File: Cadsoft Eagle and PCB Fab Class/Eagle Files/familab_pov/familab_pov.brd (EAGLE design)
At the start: 58.4 x 42.9 mm, 7 parts, among them U1 Tiny85-20-SMT

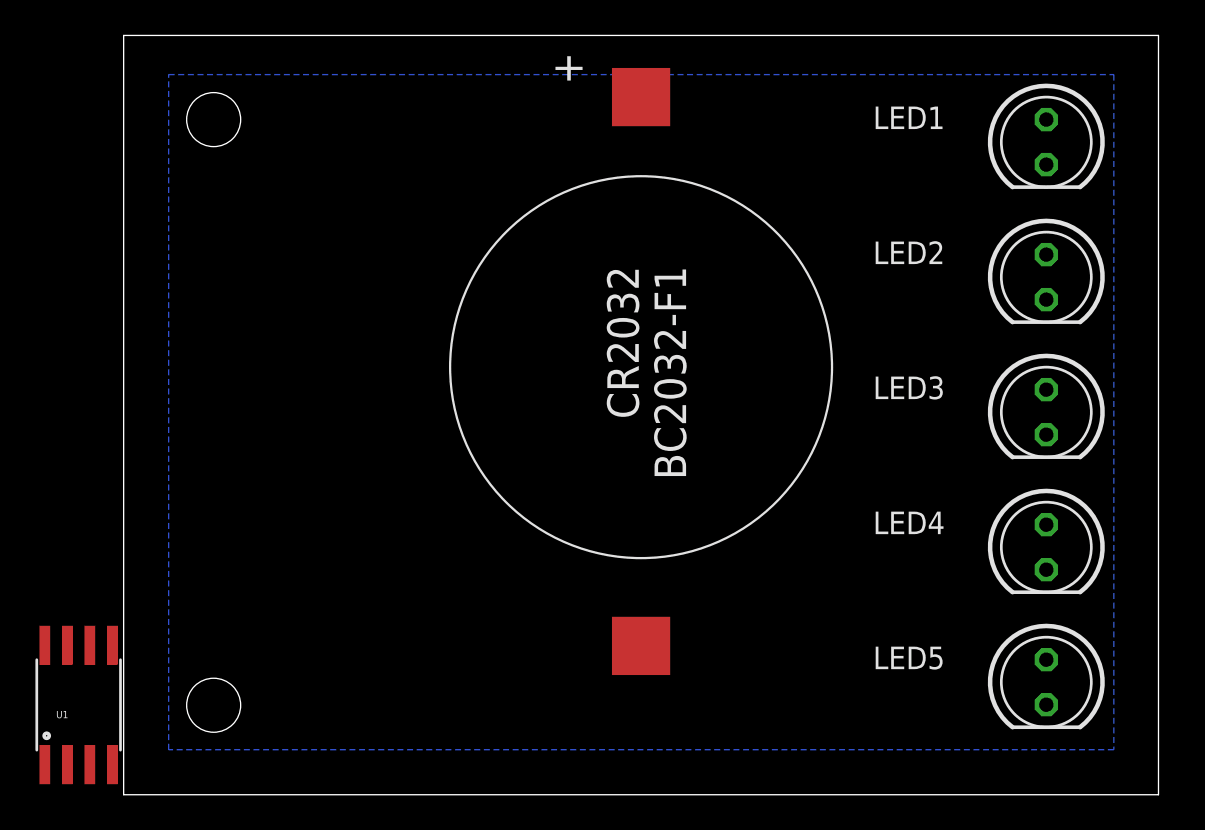
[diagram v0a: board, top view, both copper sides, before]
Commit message: Updates
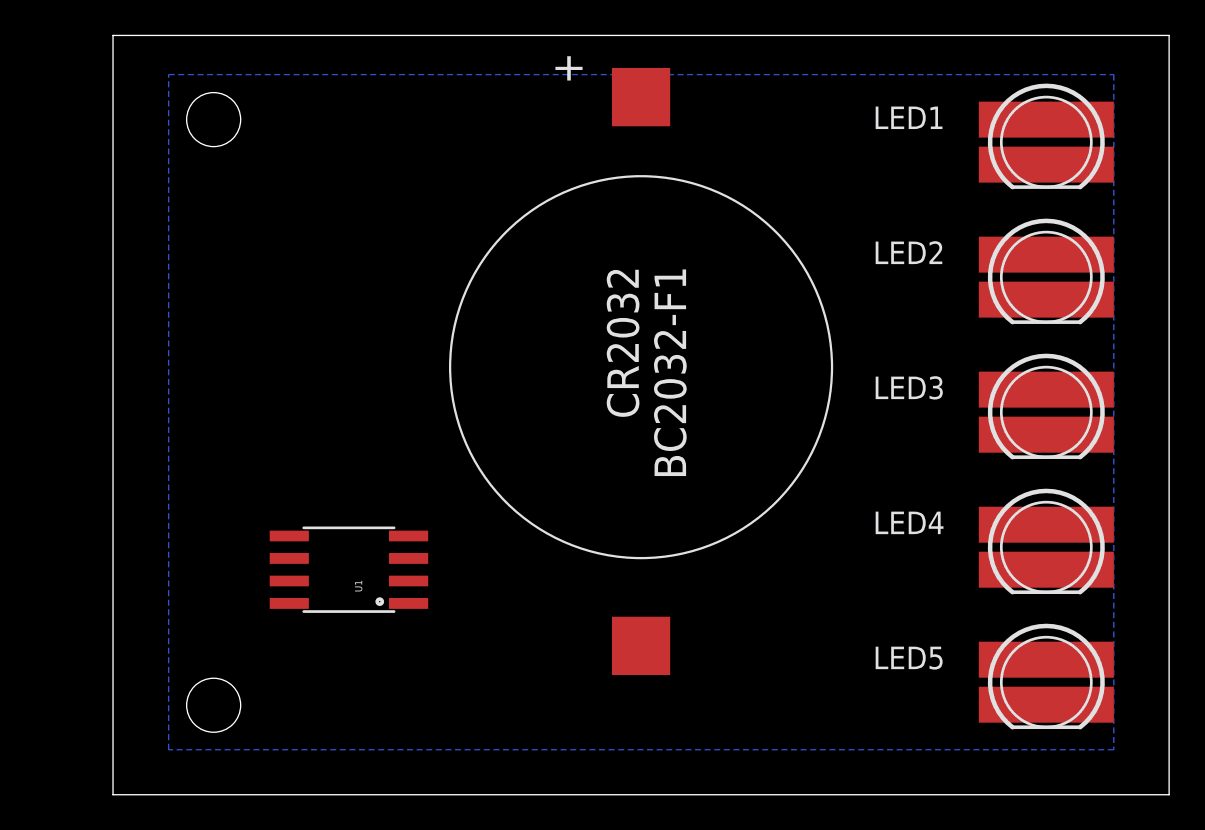
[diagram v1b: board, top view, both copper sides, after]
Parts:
- LED1, LED2, LED3, LED4, LED5: device led:LED5MM -> led:LED5MM_SMD_SIDE
- moved U1 17.0 mm to (12.7, 12.7), turned to 90 degrees
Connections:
- net N$1 renamed PB0
- net N$7 renamed PB5
- removed net N$10: LED5.A
- removed net N$2: U1.6
- removed net N$3: LED1.A
- removed net N$4: U1.7
- removed net N$5: U1.2
- removed net N$6: U1.3
- removed net N$8: LED2.A
- removed net N$9: LED4.A
- new net PB1: LED2.A, U1.6
- new net PB2: LED1.A, U1.7
- new net PB3: LED5.A, U1.2
- new net PB4: LED4.A, U1.3
- net GND: now also LED1.C, LED2.C, LED3.C, LED4.C, LED5.C; no longer LED1.K, LED2.K, LED3.K, LED4.K, LED5.K
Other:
- board size 58.4 x 42.9 mm -> 59.6 x 42.9 mm
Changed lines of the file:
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@@
 <layer number="113" name="IDFDebug" color="7" fill="1" visible="yes" active="yes"/>
 <layer number="116" name="Patch_BOT" color="9" fill="4" visible="yes" active="yes"/>
+<layer number="117" name="mPads" color="7" fill="1" visible="no" active="no"/>
+<layer number="118" name="Rect_Pads" color="7" fill="1" visible="yes" active="yes"/>
+<layer number="119" name="mUnrouted" color="7" fill="1" visible="no" active="no"/>
+<layer number="120" name="mDimension" color="7" fill="1" visible="no" active="no"/>
 <layer number="121" name="_tsilk" color="7" fill="1" visible="yes" active="yes"/>
 <layer number="122" name="_bsilk" color="7" fill="1" visible="yes" active="yes"/>
@@
 <layer number="127" name="_tValues" color="7" fill="1" visible="yes" active="yes"/>
 <layer number="128" name="_bValues" color="7" fill="1" visible="yes" active="yes"/>
+<layer number="129" name="mtStop" color="7" fill="1" visible="no" active="no"/>
+<layer number="130" name="mbStop" color="7" fill="1" visible="no" active="no"/>
 <layer number="131" name="tAdjust" color="7" fill="1" visible="yes" active="yes"/>
 <layer number="132" name="bAdjust" color="7" fill="1" visible="yes" active="yes"/>
+<layer number="133" name="mtFinish" color="7" fill="1" visible="no" active="no"/>
+<layer number="134" name="mbFinish" color="7" fill="1" visible="no" active="no"/>
+<layer number="135" name="mtGlue" color="7" fill="1" visible="no" active="no"/>
+<layer number="136" name="mbGlue" color="7" fill="1" visible="no" active="no"/>
+<layer number="137" name="mtTest" color="7" fill="1" visible="no" active="no"/>
+<layer number="138" name="mbTest" color="7" fill="1" visible="no" active="no"/>
+<layer number="139" name="mtKeepout" color="7" fill="1" visible="no" active="no"/>
+<layer number="140" name="mbKeepout" color="7" fill="1" visible="no" active="no"/>
+<layer number="141" name="mtRestrict" color="7" fill="1" visible="no" active="no"/>
+<layer number="142" name="mbRestrict" color="7" fill="1" visible="no" active="no"/>
+<layer number="143" name="mvRestrict" color="7" fill="1" visible="no" active="no"/>
 <layer number="144" name="Drill_legend" color="7" fill="1" visible="yes" active="yes"/>
+<layer number="145" name="mHoles" color="7" fill="1" visible="no" active="no"/>
+<layer number="146" name="mMilling" color="7" fill="1" visible="no" active="no"/>
+<layer number="147" name="mMeasures" color="7" fill="1" visible="no" active="no"/>
+<layer number="148" name="mDocument" color="7" fill="1" visible="no" active="no"/>
+<layer number="149" name="mReference" color="7" fill="1" visible="no" active="no"/>
 <layer number="150" name="Notes" color="7" fill="1" visible="yes" active="yes"/>
 <layer number="151" name="HeatSink" color="7" fill="1" visible="yes" active="yes"/>
@@
 <layer number="154" name="FabDoc2" color="7" fill="1" visible="yes" active="yes"/>
 <layer number="155" name="FabDoc3" color="7" fill="1" visible="yes" active="yes"/>
+<layer number="191" name="mNets" color="7" fill="1" visible="no" active="no"/>
+<layer number="192" name="mBusses" color="7" fill="1" visible="no" active="no"/>
+<layer number="193" name="mPins" color="7" fill="1" visible="no" active="no"/>
+<layer number="194" name="mSymbols" color="7" fill="1" visible="no" active="no"/>
+<layer number="195" name="mNames" color="7" fill="1" visible="no" active="no"/>
+<layer number="196" name="mValues" color="7" fill="1" visible="no" active="no"/>
 <layer number="199" name="Contour" color="7" fill="1" visible="yes" active="yes"/>
 <layer number="200" name="200bmp" color="1" fill="10" visible="yes" active="yes"/>
@@
 <layer number="223" name="223bmp" color="24" fill="1" visible="no" active="no"/>
 <layer number="224" name="224bmp" color="25" fill="1" visible="no" active="no"/>
+<layer number="231" name="Eagle3D_PG1" color="7" fill="1" visible="no" active="no"/>
+<layer number="232" name="Eagle3D_PG2" color="7" fill="1" visible="no" active="no"/>
+<layer number="233" name="Eagle3D_PG3" color="7" fill="1" visible="no" active="no"/>
 <layer number="248" name="Housing" color="7" fill="1" visible="yes" active="yes"/>
 <layer number="249" name="Edge" color="7" fill="1" visible="yes" active="yes"/>
@@
 <board>
 <plain>
-<wire x1="0" y1="0" x2="58.4" y2="0" width="0" layer="20"/>
-<wire x1="58.4" y1="0" x2="58.4" y2="42.85" width="0" layer="20"/>
-<wire x1="58.4" y1="42.85" x2="0" y2="42.85" width="0" layer="20"/>
-<wire x1="0" y1="42.85" x2="0" y2="0" width="0" layer="20"/>
+<wire x1="-0.6" y1="0" x2="59" y2="0" width="0" layer="20"/>
+<wire x1="59" y1="0" x2="59" y2="42.85" width="0" layer="20"/>
+<wire x1="59" y1="42.85" x2="-0.6" y2="42.85" width="0" layer="20"/>
+<wire x1="-0.6" y1="42.85" x2="-0.6" y2="0" width="0" layer="20"/>
 <hole x="5.08" y="5.05" drill="3.048"/>
 <hole x="5.08" y="38.1" drill="3.048"/>
@@
 </autorouter>
 <elements>
-<element name="LED1" library="led" package="LED5MM" value="" x="52.07" y="36.83" smashed="yes" rot="R270">
+<element name="LED1" library="led" package="LED5MM_SMD_SIDE" value="" x="52.07" y="36.83" smashed="yes" rot="R270">
 <attribute name="NAME" x="46.355" y="38.8366" size="1.27" layer="25" ratio="10" rot="R180"/>
 <attribute name="VALUE" x="50.2666" y="33.6296" size="1.27" layer="27" ratio="10" rot="R270"/>
 </element>
-<element name="LED2" library="led" package="LED5MM" value="" x="52.07" y="29.21" smashed="yes" rot="R270">
+<element name="LED2" library="led" package="LED5MM_SMD_SIDE" value="" x="52.07" y="29.21" smashed="yes" rot="R270">
 <attribute name="NAME" x="46.355" y="31.2166" size="1.27" layer="25" ratio="10" rot="R180"/>
 <attribute name="VALUE" x="50.2666" y="26.0096" size="1.27" layer="27" ratio="10" rot="R270"/>
 </element>
-<element name="LED3" library="led" package="LED5MM" value="" x="52.07" y="21.59" smashed="yes" rot="R270">
+<element name="LED3" library="led" package="LED5MM_SMD_SIDE" value="" x="52.07" y="21.59" smashed="yes" rot="R270">
 <attribute name="NAME" x="46.355" y="23.5966" size="1.27" layer="25" ratio="10" rot="R180"/>
 <attribute name="VALUE" x="50.2666" y="18.3896" size="1.27" layer="27" ratio="10" rot="R270"/>
 </element>
-<element name="LED4" library="led" package="LED5MM" value="" x="52.07" y="13.97" smashed="yes" rot="R270">
+<element name="LED4" library="led" package="LED5MM_SMD_SIDE" value="" x="52.07" y="13.97" smashed="yes" rot="R270">
 <attribute name="NAME" x="46.355" y="15.9766" size="1.27" layer="25" ratio="10" rot="R180"/>
 <attribute name="VALUE" x="50.2666" y="10.7696" size="1.27" layer="27" ratio="10" rot="R270"/>
 </element>
-<element name="LED5" library="led" package="LED5MM" value="" x="52.07" y="6.35" smashed="yes" rot="R270">
+<element name="LED5" library="led" package="LED5MM_SMD_SIDE" value="" x="52.07" y="6.35" smashed="yes" rot="R270">
 <attribute name="NAME" x="46.355" y="8.3566" size="1.27" layer="25" ratio="10" rot="R180"/>
 <attribute name="VALUE" x="50.2666" y="3.1496" size="1.27" layer="27" ratio="10" rot="R270"/>
 </element>
 <element name="U$1" library="pov_class" package="CR2032_BC2032-F1" value="CR2032_HOLDER" x="29.2" y="39.37" rot="R270"/>
-<element name="U1" library="SparkFun-DigitalIC" package="SO08-EIAJ" value="Tiny85-20-SMT" x="-2.54" y="5.08">
-<attribute name="PROD_ID" value="IC-09092" x="-2.54" y="5.08" size="1.778" layer="27" display="off"/>
+<element name="U1" library="SparkFun-DigitalIC" package="SO08-EIAJ" value="Tiny85-20-SMT" x="12.7" y="12.7" rot="R90">
+<attribute name="PROD_ID" value="IC-09092" x="12.7" y="12.7" size="1.778" layer="27" rot="R90" display="off"/>
 </element>
 </elements>
 <signals>
 <signal name="GND">
-<contactref element="LED1" pad="K"/>
-<contactref element="LED2" pad="K"/>
-<contactref element="LED3" pad="K"/>
-<contactref element="LED4" pad="K"/>
-<contactref element="LED5" pad="K"/>
+<contactref element="LED1" pad="C"/>
+<contactref element="LED2" pad="C"/>
+<contactref element="LED3" pad="C"/>
+<contactref element="LED4" pad="C"/>
+<contactref element="LED5" pad="C"/>
 <polygon width="0.4064" layer="16">
 <vertex x="2.54" y="40.64"/>
@@
 <contactref element="U$1" pad="POS"/>
 </signal>
-<signal name="N$1">
+<signal name="PB0">
 <contactref element="U1" pad="5"/>
 <contactref element="LED3" pad="A"/>
-<wire x1="-0.635" y1="8.4328" x2="52.07" y2="22.86" width="0" layer="19" extent="1-1"/>
-</signal>
-<signal name="N$2">
+<wire x1="9.3472" y1="14.605" x2="52.07" y2="22.86" width="0" layer="19" extent="1-1"/>
+</signal>
+<signal name="PB1">
 <contactref element="U1" pad="6"/>
-</signal>
-<signal name="N$3">
+<contactref element="LED2" pad="A"/>
+<wire x1="9.3472" y1="13.335" x2="52.07" y2="30.48" width="0" layer="19" extent="1-1"/>
+</signal>
+<signal name="PB2">
+<contactref element="U1" pad="7"/>
 <contactref element="LED1" pad="A"/>
-</signal>
-<signal name="N$4">
-<contactref element="U1" pad="7"/>
-</signal>
-<signal name="N$5">
+<wire x1="9.3472" y1="12.065" x2="52.07" y2="38.1" width="0" layer="19" extent="1-1"/>
+</signal>
+<signal name="PB3">
 <contactref element="U1" pad="2"/>
-</signal>
-<signal name="N$6">
+<contactref element="LED5" pad="A"/>
+<wire x1="16.0782" y1="12.065" x2="52.07" y2="7.62" width="0" layer="19" extent="1-1"/>
+</signal>
+<signal name="PB4">
 <contactref element="U1" pad="3"/>
-</signal>
-<signal name="N$7">
+<contactref element="LED4" pad="A"/>
+<wire x1="16.0782" y1="13.335" x2="52.07" y2="15.24" width="0" layer="19" extent="1-1"/>
+</signal>
+<signal name="PB5">
 <contactref element="U1" pad="1"/>
 </signal>
-<signal name="N$8">
-<contactref element="LED2" pad="A"/>
-</signal>
-<signal name="N$9">
-<contactref element="LED4" pad="A"/>
-</signal>
-<signal name="N$10">
-<contactref element="LED5" pad="A"/>
-</signal>
 </signals>
